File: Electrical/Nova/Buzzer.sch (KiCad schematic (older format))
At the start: 2 parts, among them IC101 74HC2GU04GW,125

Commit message: Organized the schematic
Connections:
- net labels added: BUZZER
- net labels removed: Vin
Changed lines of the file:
@@
 $Descr A4 11693 8268
 encoding utf-8
-Sheet 2 13
+Sheet 13 13
 Title ""
 Date ""
@@
 Wire Wire Line
 	6500 3700 5650 3700
-Text GLabel 4700 3100 0    50   Input ~ 0
-Vin
 Wire Wire Line
 	4700 3100 4950 3100
@@
 Wire Wire Line
 	6100 3200 6150 3200
+Text HLabel 4700 3100 0    50   Input ~ 0
+BUZZER
 $EndSCHEMATC

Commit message: Added Gyroscope
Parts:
- IC101: symbol 74HC2GU04GW_125:74HC2GU04GW,125 -> Nova-rescue:74HC2GU04GW,125-74HC2GU04GW_125
- LS101: symbol PS1440P02BT:PS1440P02BT -> Nova-rescue:PS1440P02BT-PS1440P02BT
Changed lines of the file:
@@
 $Descr A4 11693 8268
 encoding utf-8
-Sheet 13 13
+Sheet 13 14
 Title ""
 Date ""
@@
 $EndDescr
 $Comp
-L PS1440P02BT:PS1440P02BT LS101
+L Nova-rescue:PS1440P02BT-PS1440P02BT LS101
 U 1 1 5F404605
 P 5450 3800
@@
 $EndComp
 $Comp
-L 74HC2GU04GW_125:74HC2GU04GW,125 IC101
+L Nova-rescue:74HC2GU04GW,125-74HC2GU04GW_125 IC101
 U 1 1 5F40586B
 P 4950 3100

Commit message: Added Gyro pins. Organized Schematic
Need to determine if we need the interrupt pins for the sensors.
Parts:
- IC101: symbol Nova-rescue:74HC2GU04GW,125-74HC2GU04GW_125 -> Nova-rescue:74HC2GU04GW,125-74HC2GU04GW_125-Nova-rescue
- LS101: symbol Nova-rescue:PS1440P02BT-PS1440P02BT -> Nova-rescue:PS1440P02BT-PS1440P02BT-Nova-rescue
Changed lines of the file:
@@
 $EndDescr
 $Comp
-L Nova-rescue:PS1440P02BT-PS1440P02BT LS101
+L Nova-rescue:PS1440P02BT-PS1440P02BT-Nova-rescue LS101
 U 1 1 5F404605
 P 5450 3800
@@
 $EndComp
 $Comp
-L Nova-rescue:74HC2GU04GW,125-74HC2GU04GW_125 IC101
+L Nova-rescue:74HC2GU04GW,125-74HC2GU04GW_125-Nova-rescue IC101
 U 1 1 5F40586B
 P 4950 3100

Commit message: Added Pyro Channels
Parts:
- IC101: symbol Nova-rescue:74HC2GU04GW,125-74HC2GU04GW_125-Nova-rescue -> Nova-rescue:74HC2GU04GW,125-74HC2GU04GW_125-Nova-rescue-Nova-rescue
- LS101: symbol Nova-rescue:PS1440P02BT-PS1440P02BT-Nova-rescue -> Nova-rescue:PS1440P02BT-PS1440P02BT-Nova-rescue-Nova-rescue
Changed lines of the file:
@@
 $Descr A4 11693 8268
 encoding utf-8
-Sheet 13 14
+Sheet 13 16
 Title ""
 Date ""
@@
 $EndDescr
 $Comp
-L Nova-rescue:PS1440P02BT-PS1440P02BT-Nova-rescue LS101
+L Nova-rescue:PS1440P02BT-PS1440P02BT-Nova-rescue-Nova-rescue LS101
 U 1 1 5F404605
 P 5450 3800
@@
 $EndComp
 $Comp
-L Nova-rescue:74HC2GU04GW,125-74HC2GU04GW_125-Nova-rescue IC101
+L Nova-rescue:74HC2GU04GW,125-74HC2GU04GW_125-Nova-rescue-Nova-rescue IC101
 U 1 1 5F40586B
 P 4950 3100

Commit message: Added LED sheet and pins
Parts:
- IC101: symbol Nova-rescue:74HC2GU04GW,125-74HC2GU04GW_125-Nova-rescue-Nova-rescue -> Nova-rescue:74HC2GU04GW,125-74HC2GU04GW_125-Nova-rescue-Nova-rescue-Nova-rescue
- LS101: symbol Nova-rescue:PS1440P02BT-PS1440P02BT-Nova-rescue-Nova-rescue -> Nova-rescue:PS1440P02BT-PS1440P02BT-Nova-rescue-Nova-rescue-Nova-rescue
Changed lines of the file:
@@
 $Descr A4 11693 8268
 encoding utf-8
-Sheet 13 16
+Sheet 13 18
 Title ""
 Date ""
@@
 $EndDescr
 $Comp
-L Nova-rescue:PS1440P02BT-PS1440P02BT-Nova-rescue-Nova-rescue LS101
+L Nova-rescue:PS1440P02BT-PS1440P02BT-Nova-rescue-Nova-rescue-Nova-rescue LS101
 U 1 1 5F404605
 P 5450 3800
@@
 $EndComp
 $Comp
-L Nova-rescue:74HC2GU04GW,125-74HC2GU04GW_125-Nova-rescue-Nova-rescue IC101
+L Nova-rescue:74HC2GU04GW,125-74HC2GU04GW_125-Nova-rescue-Nova-rescue-Nova-rescue IC101
 U 1 1 5F40586B
 P 4950 3100
+AR Path="/5F40586B" Ref="IC101"  Part="1"
+AR Path="/5F36176A/5F40586B" Ref="IC101"  Part="1"
 F 0 "IC101" H 5450 3365 50  0000 C CNN
 F 1 "74HC2GU04GW,125" H 5450 3274 50  0000 C CNN

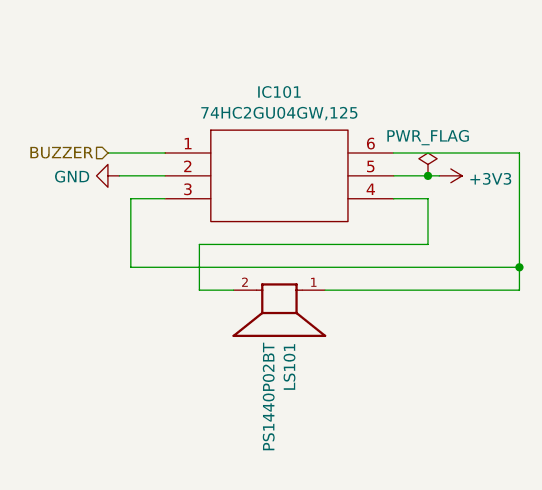
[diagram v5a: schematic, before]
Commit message: Minor update
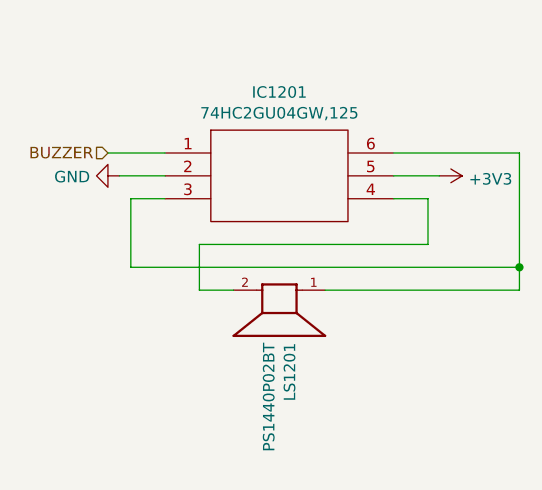
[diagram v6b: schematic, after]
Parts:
- renumbered IC101 to IC1201, LS101 to LS1201
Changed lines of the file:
@@
 $Descr A4 11693 8268
 encoding utf-8
-Sheet 13 18
+Sheet 12 18
 Title ""
 Date ""
@@
 $EndDescr
 $Comp
-L Nova-rescue:PS1440P02BT-PS1440P02BT-Nova-rescue-Nova-rescue-Nova-rescue LS101
+L Nova-rescue:PS1440P02BT-PS1440P02BT-Nova-rescue-Nova-rescue-Nova-rescue LS1201
 U 1 1 5F404605
 P 5450 3800
-F 0 "LS101" H 5580 3846 50  0000 L CNN
+F 0 "LS1201" H 5580 3846 50  0000 L CNN
 F 1 "PS1440P02BT" H 5580 3755 50  0000 L CNN
 F 2 "Footprint Library:BUZZER_PS1440P02BT" H 5450 3800 50  0001 L BNN
@@
 $EndComp
 $Comp
-L Nova-rescue:74HC2GU04GW,125-74HC2GU04GW_125-Nova-rescue-Nova-rescue-Nova-rescue IC101
+L Nova-rescue:74HC2GU04GW,125-74HC2GU04GW_125-Nova-rescue-Nova-rescue-Nova-rescue IC?
 U 1 1 5F40586B
 P 4950 3100
-AR Path="/5F40586B" Ref="IC101"  Part="1"
-AR Path="/5F36176A/5F40586B" Ref="IC101"  Part="1"
-F 0 "IC101" H 5450 3365 50  0000 C CNN
+AR Path="/5F40586B" Ref="IC?"  Part="1"
+AR Path="/5F36176A/5F40586B" Ref="IC1201"  Part="1"
+F 0 "IC1201" H 5450 3365 50  0000 C CNN
 F 1 "74HC2GU04GW,125" H 5450 3274 50  0000 C CNN
 F 2 "Footprint Library:SOP65P210X110-6N" H 5800 3200 50  0001 L CNN
@@
 $EndComp
 $Comp
-L power:GND #PWR0101
+L power:GND #PWR01201
 U 1 1 5F407098
 P 4750 3200
-F 0 "#PWR0101" H 4750 2950 50  0001 C CNN
+F 0 "#PWR01201" H 4750 2950 50  0001 C CNN
 F 1 "GND" V 4755 3072 50  0000 R CNN
 F 2 "" H 4750 3200 50  0001 C CNN
@@
 	4950 3200 4750 3200
 $Comp
-L power:+3V3 #PWR0102
+L power:+3V3 #PWR01202
 U 1 1 5F4096B6
 P 6150 3200
-F 0 "#PWR0102" H 6150 3050 50  0001 C CNN
+F 0 "#PWR01202" H 6150 3050 50  0001 C CNN
 F 1 "+3V3" V 6165 3328 50  0000 L CNN
 F 2 "" H 6150 3200 50  0001 C CNN
@@
 	0    1    1    0
 $EndComp
-Wire Wire Line
-	5950 3200 6100 3200
 Wire Wire Line
 	5950 3100 6500 3100
@@
 Wire Wire Line
 	6500 3600 6500 3700
-$Comp
-L power:PWR_FLAG #FLG0101
-U 1 1 5F410118
-P 6100 3200
-F 0 "#FLG0101" H 6100 3275 50  0001 C CNN
-F 1 "PWR_FLAG" H 6100 3373 50  0000 C CNN
-F 2 "" H 6100 3200 50  0001 C CNN
-F 3 "~" H 6100 3200 50  0001 C CNN
-	1    6100 3200
-	1    0    0    -1
-$EndComp
-Connection ~ 6100 3200
-Wire Wire Line
-	6100 3200 6150 3200
 Text HLabel 4700 3100 0    50   Input ~ 0
 BUZZER
+Wire Wire Line
+	5950 3200 6150 3200
 $EndSCHEMATC

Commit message: Added Accelerometer
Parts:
- IC1201: symbol Nova-rescue:74HC2GU04GW,125-74HC2GU04GW_125-Nova-rescue-Nova-rescue-Nova-rescue -> Nova-rescue:74HC2GU04GW,125-74HC2GU04GW_125-Nova-rescue-Nova-rescue-Nova-rescue-Nova-rescue
- LS1201: symbol Nova-rescue:PS1440P02BT-PS1440P02BT-Nova-rescue-Nova-rescue-Nova-rescue -> Nova-rescue:PS1440P02BT-PS1440P02BT-Nova-rescue-Nova-rescue-Nova-rescue-Nova-rescue
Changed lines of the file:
@@
 $Descr A4 11693 8268
 encoding utf-8
-Sheet 12 18
+Sheet 12 19
 Title ""
 Date ""
@@
 $EndDescr
 $Comp
-L Nova-rescue:PS1440P02BT-PS1440P02BT-Nova-rescue-Nova-rescue-Nova-rescue LS1201
+L Nova-rescue:PS1440P02BT-PS1440P02BT-Nova-rescue-Nova-rescue-Nova-rescue-Nova-rescue LS1201
 U 1 1 5F404605
 P 5450 3800
@@
 $EndComp
 $Comp
-L Nova-rescue:74HC2GU04GW,125-74HC2GU04GW_125-Nova-rescue-Nova-rescue-Nova-rescue IC?
+L Nova-rescue:74HC2GU04GW,125-74HC2GU04GW_125-Nova-rescue-Nova-rescue-Nova-rescue-Nova-rescue IC?
 U 1 1 5F40586B
 P 4950 3100

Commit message: Fixed File paths for 0603
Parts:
- IC1201: symbol Nova-rescue:74HC2GU04GW,125-74HC2GU04GW_125-Nova-rescue-Nova-rescue-Nova-rescue-Nova-rescue -> Nova-rescue:74HC2GU04GW,125-74HC2GU04GW_125-Nova-rescue-Nova-rescue-Nova-rescue-Nova-rescue-Nova-rescue
- LS1201: symbol Nova-rescue:PS1440P02BT-PS1440P02BT-Nova-rescue-Nova-rescue-Nova-rescue-Nova-rescue -> Nova-rescue:PS1440P02BT-PS1440P02BT-Nova-rescue-Nova-rescue-Nova-rescue-Nova-rescue-Nova-rescue
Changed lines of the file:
@@
 $EndDescr
 $Comp
-L Nova-rescue:PS1440P02BT-PS1440P02BT-Nova-rescue-Nova-rescue-Nova-rescue-Nova-rescue LS1201
+L Nova-rescue:PS1440P02BT-PS1440P02BT-Nova-rescue-Nova-rescue-Nova-rescue-Nova-rescue-Nova-rescue LS1201
 U 1 1 5F404605
 P 5450 3800
@@
 $EndComp
 $Comp
-L Nova-rescue:74HC2GU04GW,125-74HC2GU04GW_125-Nova-rescue-Nova-rescue-Nova-rescue-Nova-rescue IC?
+L Nova-rescue:74HC2GU04GW,125-74HC2GU04GW_125-Nova-rescue-Nova-rescue-Nova-rescue-Nova-rescue-Nova-rescue IC?
 U 1 1 5F40586B
 P 4950 3100
